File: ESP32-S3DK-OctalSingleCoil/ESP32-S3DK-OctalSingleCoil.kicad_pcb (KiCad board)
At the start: 2 copper layers, 41 parts, among them J301 RJ45, J302 RJ45, J501 - 12-15 +, J502 Motor 1, J503 Motor 2, J504 Motor 4, J505 Motor 3, J506 Motor 5, J507 Motor 6, J508 Motor 8, J509 Motor 7, T301 - 15 in +, T302 - 15 out +, U301 TCAN332DR, U401 AP63205, U501 TC4427, U502 TC4427, U503 TC4427, U504 TC4427

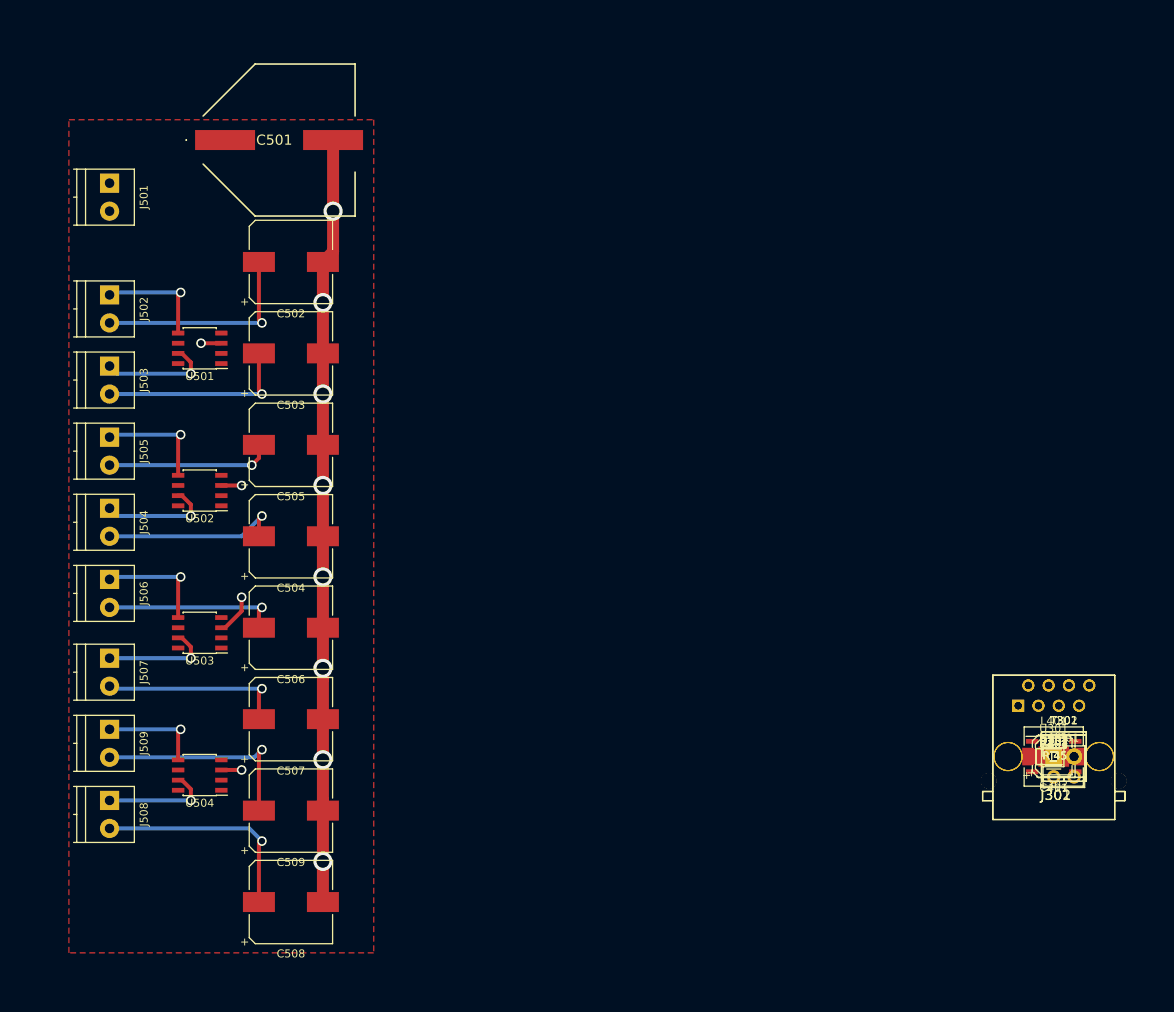
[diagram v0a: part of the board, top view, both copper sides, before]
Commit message: Almost done with ESP32-S3DK-OctalSingleCoil.
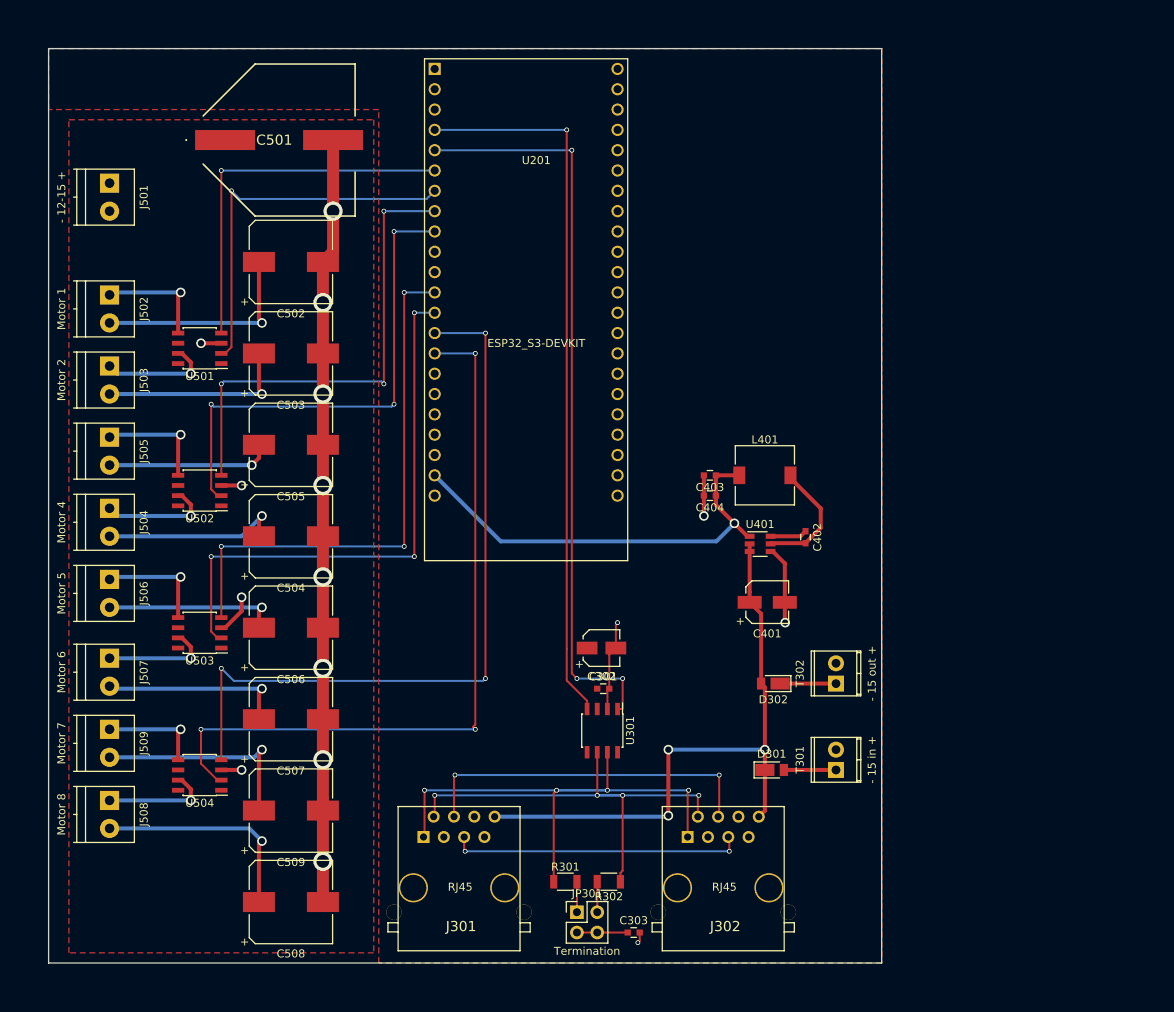
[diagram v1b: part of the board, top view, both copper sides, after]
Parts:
- added U201: ESP32_S3-DEVKIT, ESP32-S3-Devkit-C, F.Cu at (83.8, 41.9)
- moved J301 76.1 mm to (74.2, 121.4)
- moved R301 63.0 mm to (87.5, 120.7)
- moved JP301 62.7 mm to (88.9, 124.5)
- moved C302 58.1 mm to (92.0, 91.4)
- moved R302 57.8 mm to (92.9, 120.7), turned to 180 degrees
- moved C301 56.9 mm to (92.2, 96.5)
- moved C303 56.9 mm to (96.0, 127.0)
- moved U301 56.5 mm to (92.1, 101.8), turned to 270 degrees
- moved C403 55.5 mm to (105.5, 69.8), turned to 180 degrees
- moved C404 53.9 mm to (105.5, 72.4), turned to 180 degrees
- moved L401 50.4 mm to (112.4, 69.8)
- moved U401 45.3 mm to (111.8, 78.4)
- moved J302 44.5 mm to (107.2, 121.4)
- moved C402 41.4 mm to (117.5, 77.6), turned to 270 degrees
- moved C401 40.7 mm to (112.7, 85.7)
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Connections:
- U501 pad 2: /Octal Single Coil Switch Machine/Motor_2 -> /MCU/GPIO7/Motor2
- U501 pad 4: /Octal Single Coil Switch Machine/Motor_1 -> /MCU/GPIO6/Motor1
- U502 pad 2: /Octal Single Coil Switch Machine/Motor_4 -> /MCU/GPIO16/Motor4
- U502 pad 4: /Octal Single Coil Switch Machine/Motor_3 -> /MCU/GPIO15/Motor3
- U503 pad 2: /Octal Single Coil Switch Machine/Motor_6 -> /MCU/GPIO3/Motor6
- U503 pad 4: /Octal Single Coil Switch Machine/Motor_5 -> /MCU/GPIO8/Motor5
- U504 pad 2: /Octal Single Coil Switch Machine/Motor_8 -> /MCU/GPIO9/Motor8
- U504 pad 4: /Octal Single Coil Switch Machine/Motor_7 -> /MCU/GPIO46/Motor7
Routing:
- net /MCU/GPIO46/Motor7: track 0.00 -> 94.8 mm, vias 0 -> 3
- net /MCU/GPIO9/Motor8: track 0.00 -> 94.3 mm, vias 0 -> 3
- net /CAN Transciver/CAN_TX: track 0.00 -> 93.6 mm, vias 0 -> 3
- net /CAN Transciver/CAN_RX: track 0.00 -> 90.0 mm, vias 0 -> 1
- net CAN +12V: track 0.00 -> 77.3 mm, vias 0 -> 3
- net /MCU/GPIO3/Motor6: track 0.00 -> 69.4 mm, vias 0 -> 3
- net /CAN Transciver/CANH: track 0.00 -> 67.5 mm, vias 0 -> 4
- net /MCU/GPIO8/Motor5: track 0.00 -> 67.3 mm, vias 0 -> 3
- net /MCU/GPIO16/Motor4: track 0.00 -> 62.0 mm, vias 0 -> 3
- net /MCU/GPIO15/Motor3: track 0.00 -> 59.9 mm, vias 0 -> 3
- net /CAN Transciver/CANL: track 0.00 -> 57.9 mm, vias 0 -> 4
- net +5V: track 0.00 -> 54.3 mm, vias 0 -> 1
- net /MCU/GPIO7/Motor2: track 0.00 -> 47.4 mm, vias 0 -> 1
- net /MCU/GPIO6/Motor1: track 0.00 -> 47.0 mm, vias 0 -> 1
- net Net-(J301-Pad4): track 0.00 -> 43.5 mm, vias 0 -> 2
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- added copper zone on F.Cu, net +3V3
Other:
- board outline added: 104.1 x 114.3 mm
